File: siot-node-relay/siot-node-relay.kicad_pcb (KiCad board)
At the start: 2 copper layers, 40.7 x 46.6 mm, 15 parts, among them J1 xConnect_smd, J2 xConnect_smd, J3 Screw_Terminal_5mm_01x03, Q1 BSS84, U1 DS2413P_, U2 ADP7142ARDZ-5.0, U3 STWD100NYWY3F

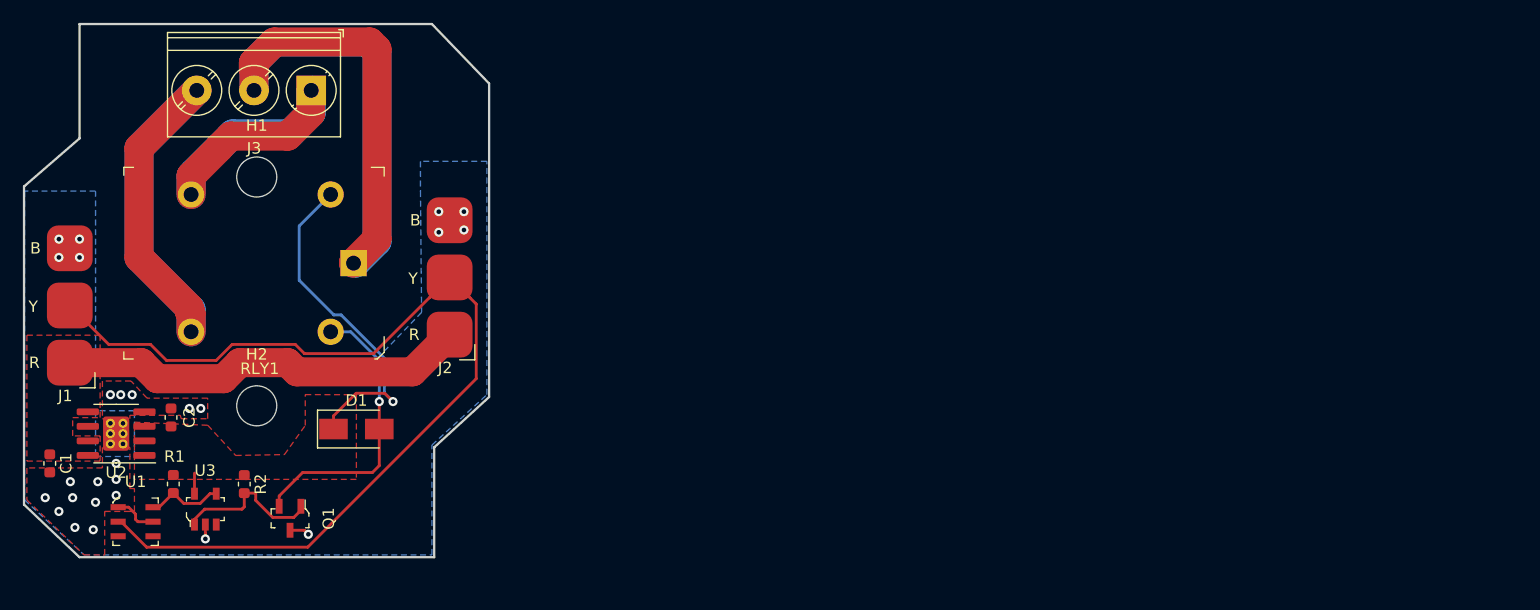
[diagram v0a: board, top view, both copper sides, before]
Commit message: redo relay node
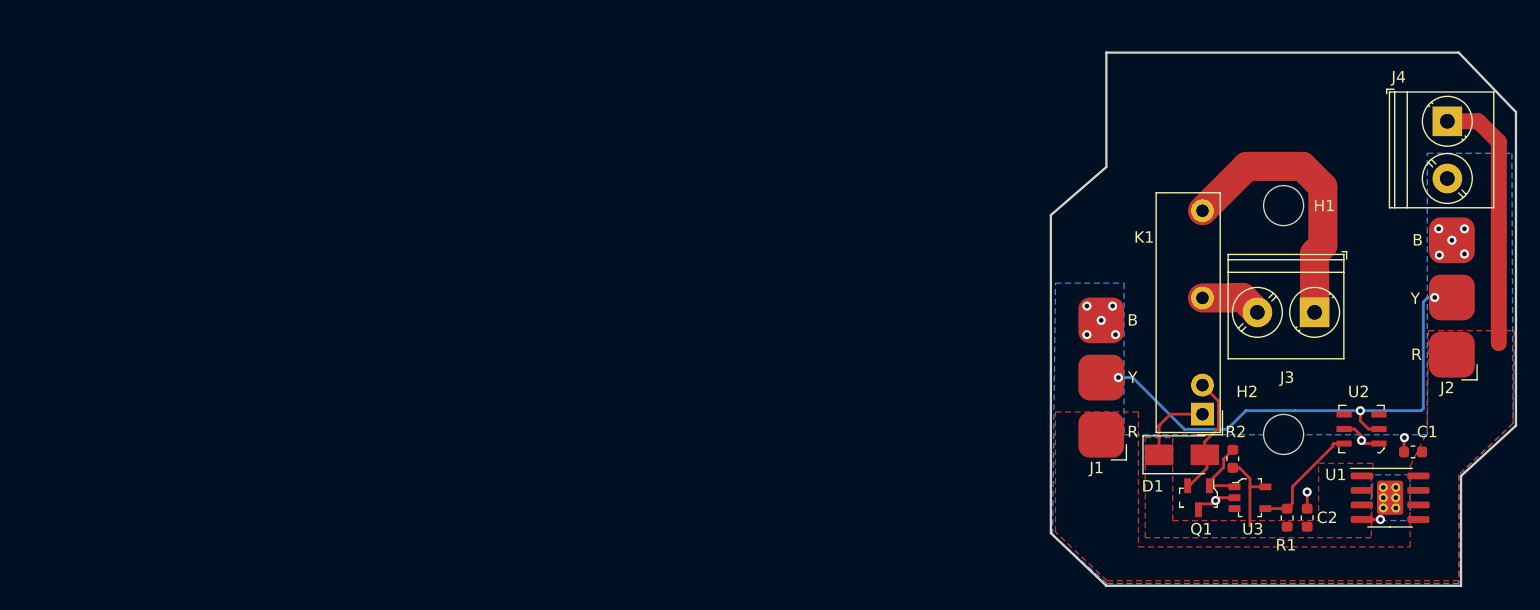
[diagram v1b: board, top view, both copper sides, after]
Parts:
- removed RLY1: G5LE-14_DC5, digikey-footprints:Relay_THT_G5LE-14
- added J4: Screw_Terminal_5mm_01x02, TerminalBlock_Phoenix:TerminalBlock_Phoenix_PT-1,5-2-5.0-H_1x02_P5.00mm_Horizontal, F.Cu at (194.8, 78.1)
- added K1: G6DN-1A-L-DC5, BEC:OMRON-G6DN-1A-L, F.Cu at (173.3, 103.7)
- J3: value Screw_Terminal_5mm_01x03 -> Screw_Terminal_5mm_01x02; footprint TerminalBlock_Phoenix:TerminalBlock_Phoenix_PT-1,5-3-5.0-H_1x03_P5.00mm_Horizontal -> TerminalBlock_Phoenix:TerminalBlock_Phoenix_PT-1,5-2-5.0-H_1x02_P5.00mm_Horizontal
- moved C1 119.2 mm to (191.8, 107.0), turned to 180 degrees
- moved U2 111.5 mm to (189.8, 111.0), turned to 0 degrees
- moved U1 107.5 mm to (187.2, 105.0), turned to 180 degrees
- moved C2 99.7 mm to (182.5, 112.8)
- moved R1 97.4 mm to (180.8, 112.8), turned to 90 degrees
- moved U3 91.3 mm to (177.5, 111.0), turned to 270 degrees
- moved J1 90.4 mm to (164.5, 105.5)
- moved J3 89.8 mm to (183.2, 94.8)
- moved H1 89.8 mm to (180.4, 85.5)
- moved H2 89.8 mm to (180.4, 105.5)
- moved J2 87.6 mm to (195.2, 98.5)
- moved R2 86.4 mm to (176.0, 107.6), turned to 90 degrees
- moved Q1 79.4 mm to (173.0, 111.0)
- moved D1 72.2 mm to (171.6, 107.2)
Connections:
- J3 pad 1: Net-(J3-Pad1) -> /relay_1
- J3 pad 2: Net-(J3-Pad2) -> /relay_2
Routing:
- net Net-(J3-Pad2): track 67.5 -> 0.00 mm
- net Net-(J3-Pad3): track 50.2 -> 0.00 mm
- net Net-(J1-PadY): track 87.4 -> 42.7 mm, vias 0 -> 3
- net Net-(J3-Pad1): track 32.8 -> 0.00 mm
- net /relay_1: track 0.00 -> 24.1 mm
- net +5V: track 32.3 -> 14.2 mm, vias 1 -> 0
- net Net-(D1-Pad2): track 25.2 -> 10.7 mm, vias 1 -> 0
- net +24V: track 36.0 -> 22.8 mm
- net Net-(Q1-Pad1): track 13.3 -> 6.23 mm
- net /relay_2: track 0.00 -> 5.36 mm
- net GND: track 6.84 -> 11.5 mm, vias 26 -> 15
- net Net-(R1-Pad2): track 6.77 -> 10.2 mm
- removed copper zone on F.Cu, net GND
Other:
- outline, holes or cut-outs redrawn
- net class relay added: clearance 0.4064, trace_width 2.54, via_dia 0.8, via_drill 0.4
